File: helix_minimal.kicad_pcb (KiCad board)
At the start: 2 copper layers, 50 x 50 mm, 20 parts, among them J1 USB-C, J4 sd card, J5 SWD, J6 pico hdmi, U1 STM32C071FBP6, U2 AP2112K-3.3, U3 WIZ850io

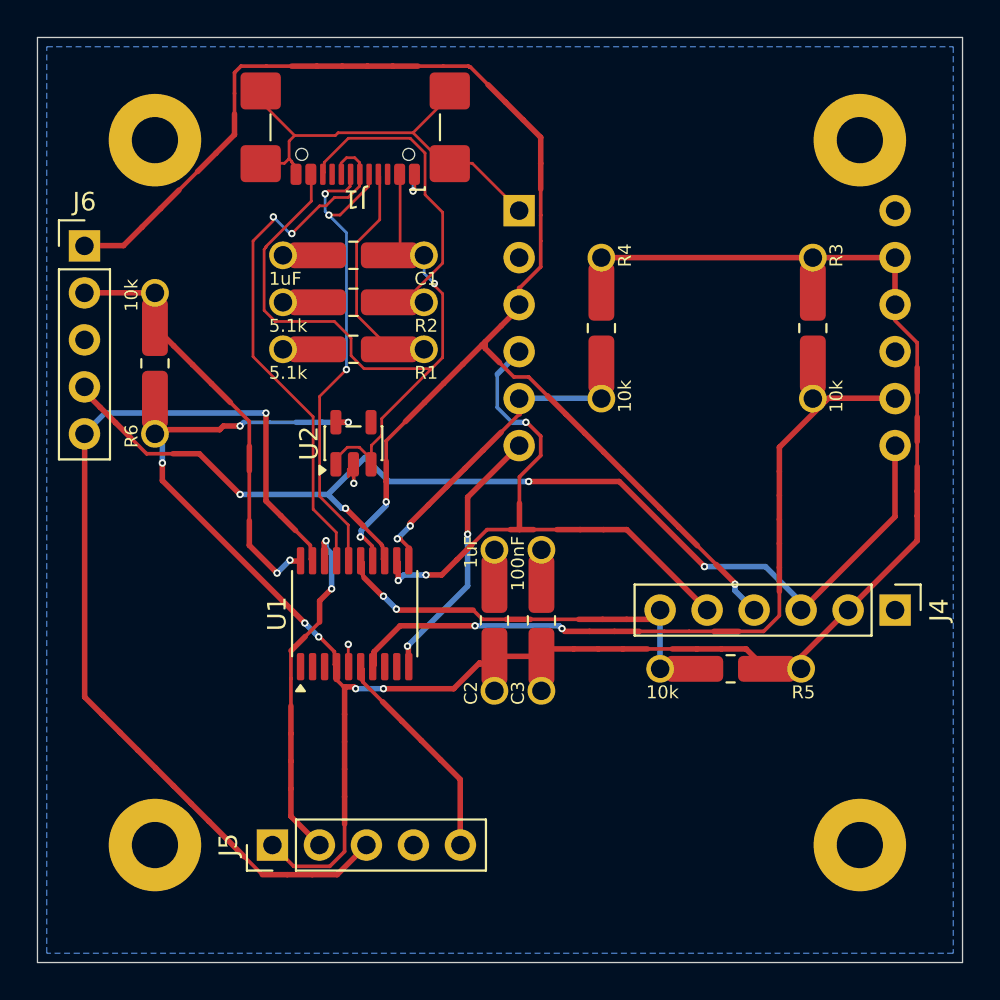
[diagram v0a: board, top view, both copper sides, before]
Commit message: Reroute board with hard 0.30 mm ordinary traces
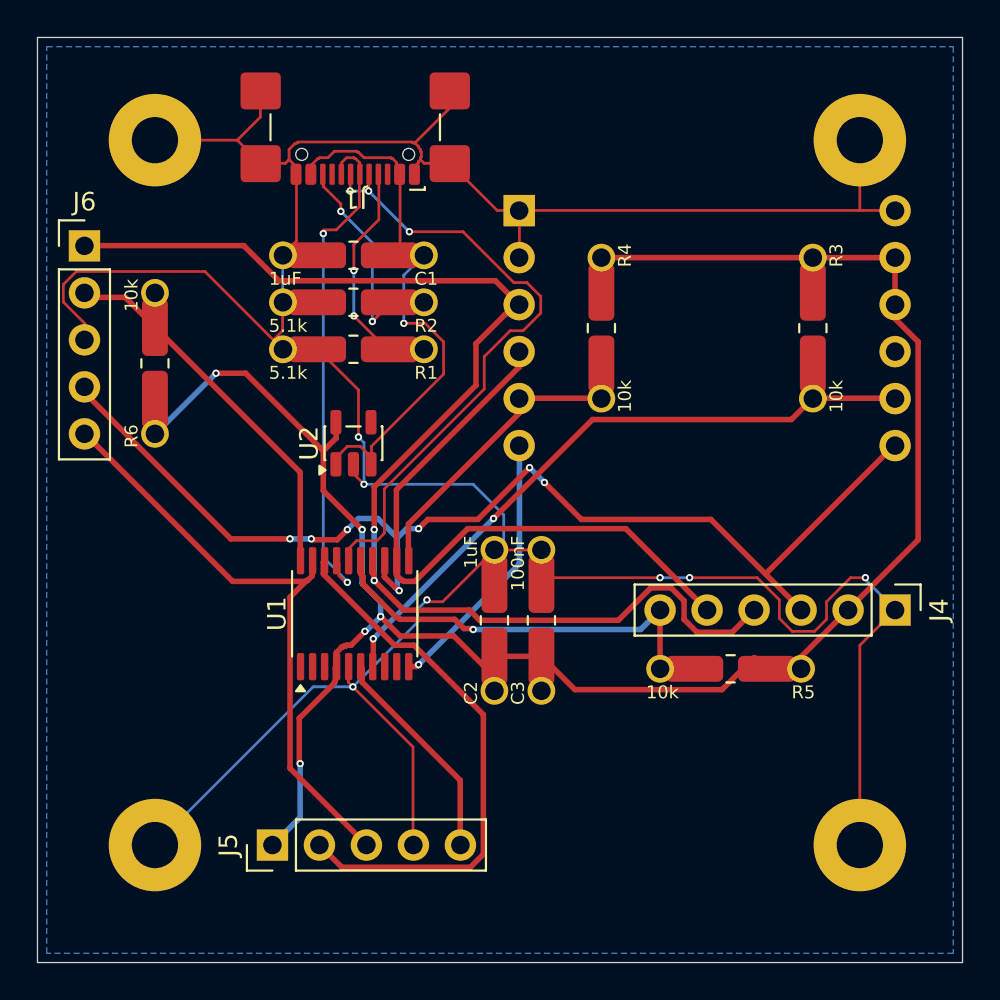
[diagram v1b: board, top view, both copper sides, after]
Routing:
- net GND: track 29.6 -> 181.3 mm, vias 3 -> 7
- net /SWCLK: track 53.4 -> 32.9 mm, vias 1 -> 0
- net VBUS: track 41.6 -> 30.4 mm
- net /SPI_MOSI: track 80.0 -> 68.9 mm, vias 3 -> 2
- net /SWDIO: track 19.3 -> 29.7 mm, vias 2 -> 0
- net /USB_DM: track 27.2 -> 34.2 mm
- net /CC2: track 17.1 -> 10.6 mm, vias 0 -> 2
- net /WIZ_RST: track 40.9 -> 35.1 mm
- net +3V3: track 107.5 -> 104.3 mm, vias 7 -> 5
- net /SPI_SCK: track 32.7 -> 34.8 mm, vias 3 -> 0
- net /USB_DP: track 29.4 -> 27.5 mm
- net /SPI_MISO: track 61.1 -> 62.6 mm, vias 4 -> 7
- net /PICO_CS: track 21.3 -> 20.1 mm, vias 2 -> 0
- net /SD_CS: track 21.2 -> 21.9 mm, vias 2 -> 1
- net /WIZ_CS: track 16.4 -> 15.7 mm, vias 2 -> 0
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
